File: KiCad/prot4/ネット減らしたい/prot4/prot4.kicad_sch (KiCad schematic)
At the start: 216 parts, among them J1 Conn_01x02_Socket, J2 LED_SW, J3 Conn_01x04_Socket, Q1 Q_Photo_NPN, Q10 Q_Photo_NPN, Q11 Q_Photo_NPN, Q12 Q_Photo_NPN, Q13 Q_Photo_NPN, Q14 Q_Photo_NPN, Q15 Q_Photo_NPN, Q16 Q_Photo_NPN, Q17 Q_Photo_NPN, Q18 Q_Photo_NPN, Q19 Q_Photo_NPN, Q2 Q_Photo_NPN, Q20 Q_Photo_NPN, Q21 Q_Photo_NPN, Q22 Q_Photo_NPN, Q23 Q_Photo_NPN, Q24 Q_Photo_NPN, Q25 Q_Photo_NPN, Q26 Q_Photo_NPN, Q27 Q_Photo_NPN, Q28 Q_Photo_NPN, Q29 Q_Photo_NPN, Q3 Q_Photo_NPN, Q30 Q_Photo_NPN, Q31 Q_Photo_NPN, Q32 Q_Photo_NPN, Q4 Q_Photo_NPN, Q5 Q_Photo_NPN, Q6 Q_Photo_NPN, Q7 Q_Photo_NPN, Q8 Q_Photo_NPN, Q9 Q_Photo_NPN, U1 LM393, U10 LM393, U11 LM393, U12 LM393, U13 LM393, U14 LM393, U15 LM393, U16 LM393, U2 LM393, U3 LM393, U4 LM393, U5 LM393, U6 LM393, U7 LM393, U8 LM393, U9 LM393

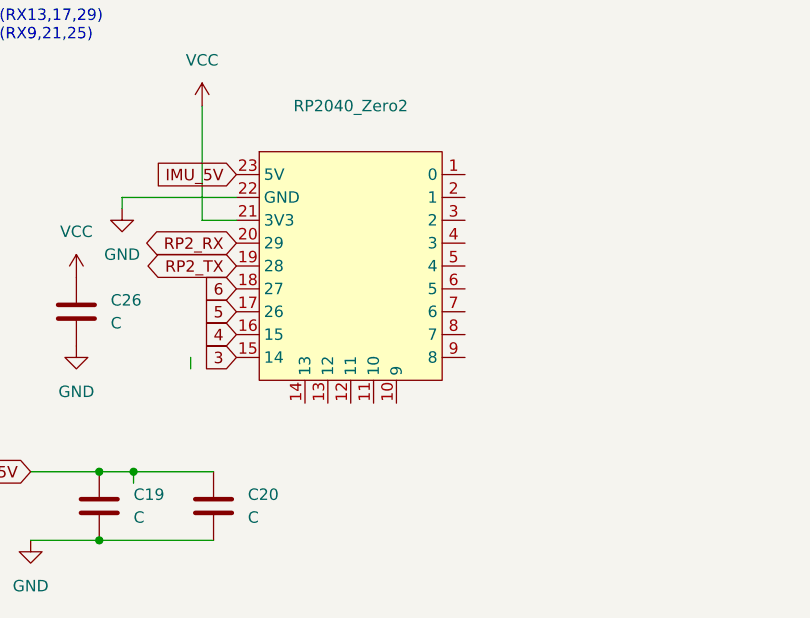
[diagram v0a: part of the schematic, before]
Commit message: 配線終了
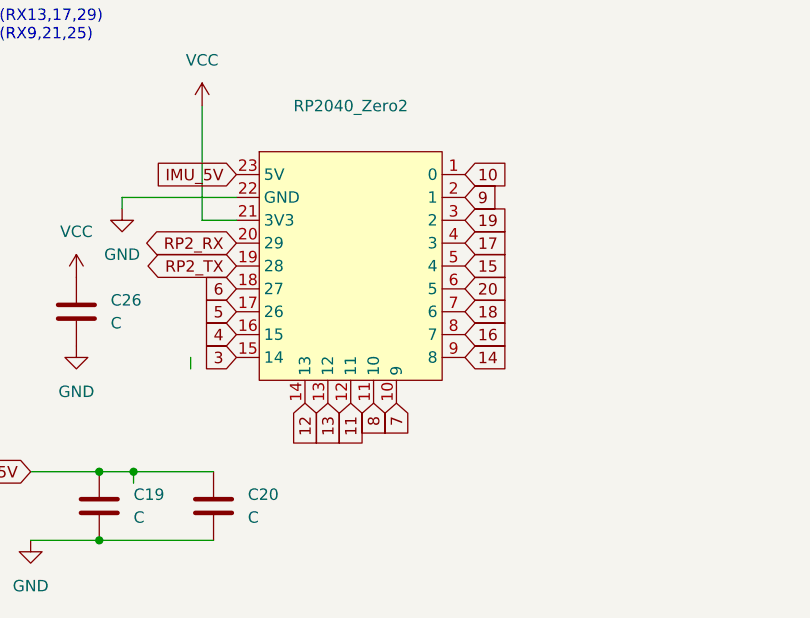
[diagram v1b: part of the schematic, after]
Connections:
- net 10: now also RP2040_Zero2.1 (0)
- net 11: now also RP2040_Zero2.12 (11)
- net 12: now also RP2040_Zero2.14 (13)
- net 13: now also RP2040_Zero2.13 (12)
- net 14: now also RP2040_Zero2.9 (8)
- net 15: now also RP2040_Zero2.5 (4)
- net 16: now also RP2040_Zero2., RP2040_Zero2.8 (7)
- net 17: now also RP2040_Zero2.4 (3)
- net 18: now also RP2040_Zero2.7 (6)
- net 19: now also RP2040_Zero2.3 (2)
- net 20: now also RP2040_Zero2.6 (5)
- net 7: now also RP2040_Zero2.10 (9)
- net 8: now also RP2040_Zero2.11 (10)
- net 9: now also RP2040_Zero2.2 (1)
